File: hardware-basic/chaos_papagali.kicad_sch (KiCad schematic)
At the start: 40 parts, among them J1 Conn_01x06, J2 USB_B_Micro, J3 BAT, M1 Motor_DC, Q1 BC847, SW1 SW_Push, SW3 SW_DIP_x04, U1 ATmega328P-M, U2 TP4056, U4 FS8205A, Y1 8MHz

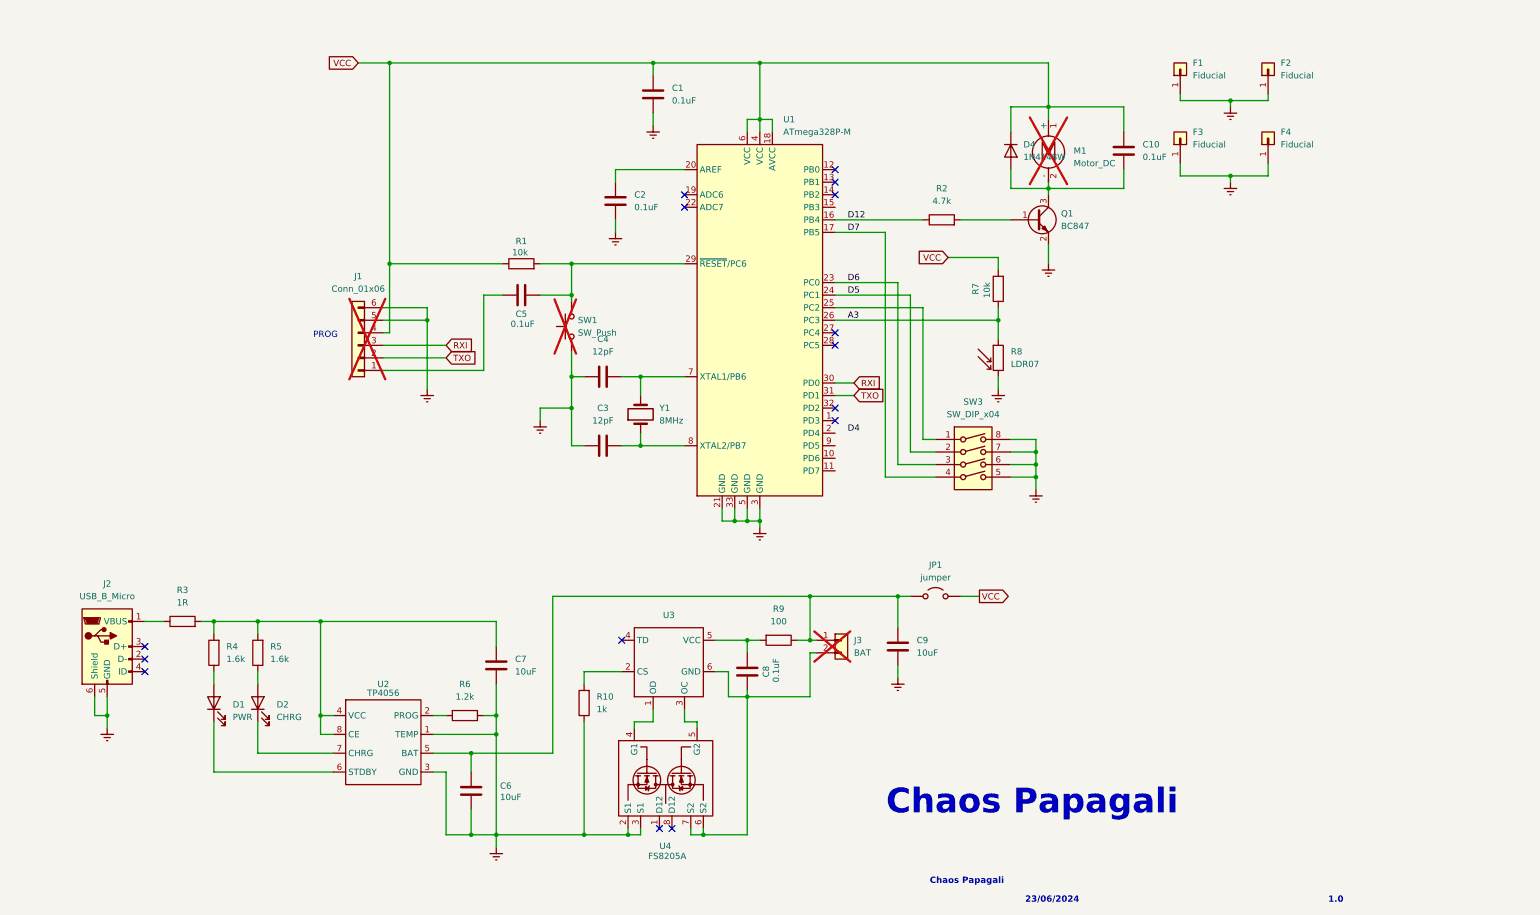
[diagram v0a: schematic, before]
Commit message: First full project commit
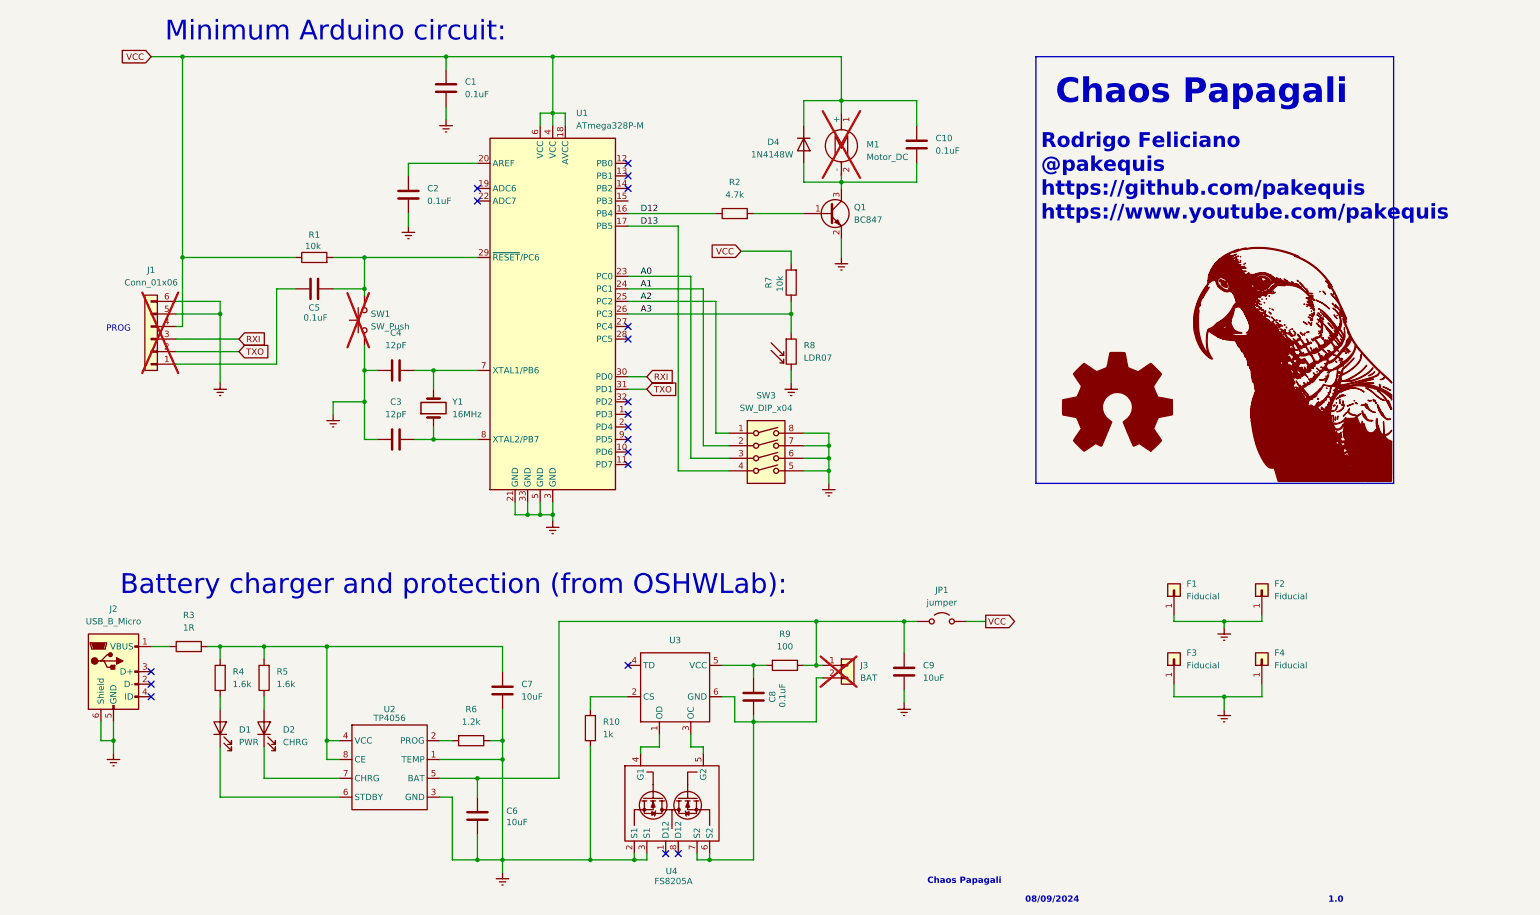
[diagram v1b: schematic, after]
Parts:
- Y1: value 8MHz -> 16MHz
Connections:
- net A2: now reaches SW3.1, U1.25 (PC2)
- net D5 renamed A1
- net D6 renamed A0
- net D7 renamed D13
- no-connect marks 15 -> 19
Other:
- note added: "08/09/2024"
- note added: "Battery charger and protection (from OSHWLab):"
- note added: "Minimum Arduino circuit:"
- note added: "Rodrigo Feliciano @pakequis https://github.com/pakequis https://www.youtube.com/pakequis"
- note removed: "23/06/2024"
- moved on the sheet: C1, C10, C2, C3, C4, C5, C6, C7, C8, C9, D1, D2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
